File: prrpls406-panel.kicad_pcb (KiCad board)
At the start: 2 copper layers, 36 x 36 mm, 384 parts, among them U1 ATtiny406-M

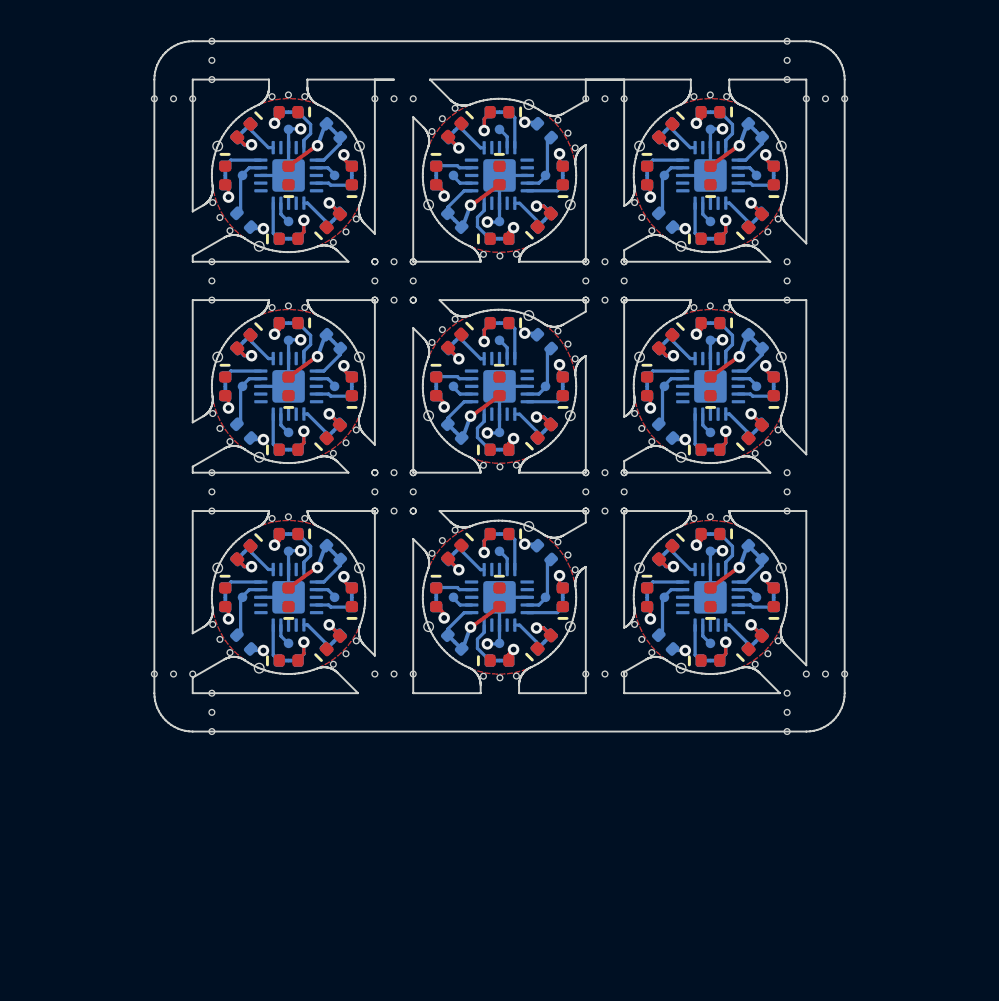
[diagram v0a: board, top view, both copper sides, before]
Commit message: submitting
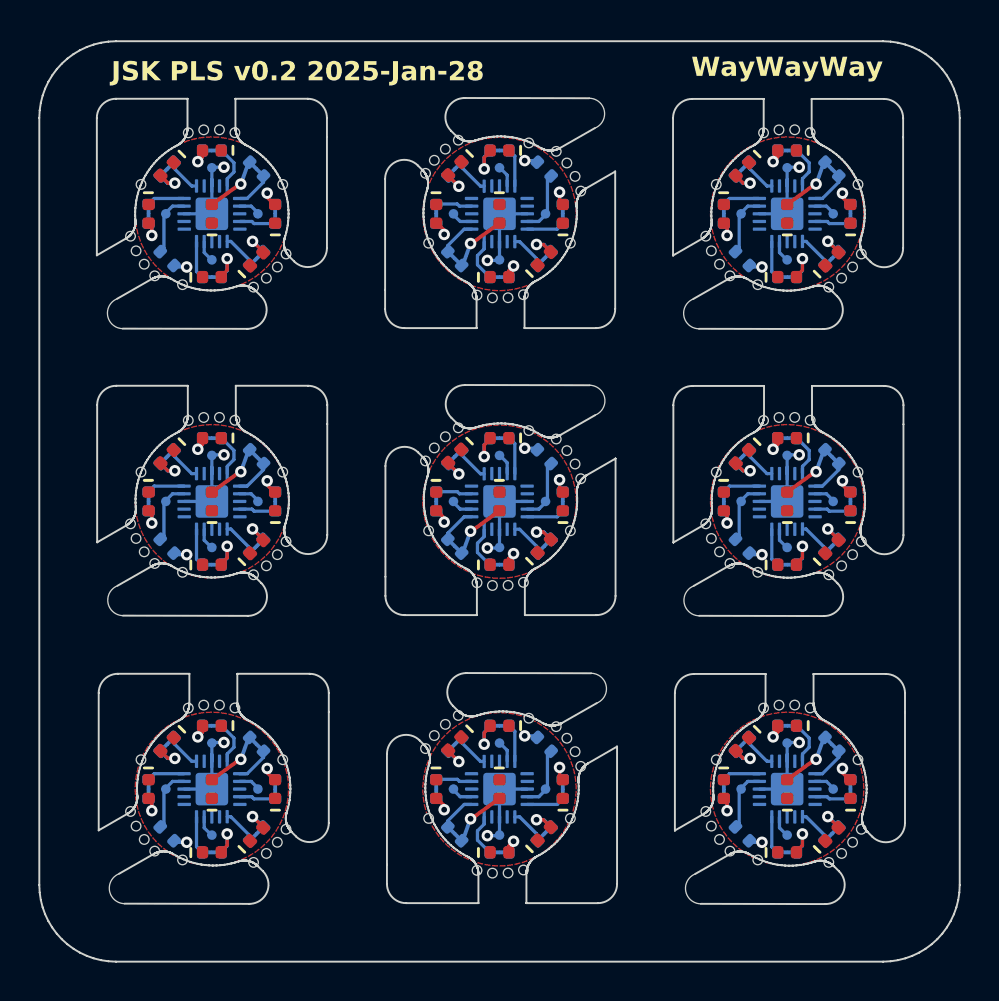
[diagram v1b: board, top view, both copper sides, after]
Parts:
- removed the C1 at (157.2, 40.3)
- removed the C1 at (150.8, 35.7)
- removed the C1 at (150.8, 46.7)
- removed the C1 at (157.2, 51.3)
- removed the C1 at (135.2, 29.3)
- removed the C1 at (135.2, 40.3)
- removed the C1 at (135.2, 51.3)
- removed the C1 at (150.8, 24.7)
- removed the C1 at (157.2, 29.3)
- removed the D1 at (159.5, 34.7)
- removed the D1 at (137.5, 34.7)
- removed the D1 at (148.5, 41.3)
- removed the D1 at (137.5, 45.7)
- removed the D1 at (159.5, 45.7)
- removed the D1 at (159.5, 23.7)
- removed the D1 at (137.5, 23.7)
- removed the D1 at (148.5, 30.3)
- removed the D1 at (148.5, 52.3)
- removed the D2 at (135.2, 24.7)
- removed the D2 at (157.2, 35.7)
- removed the D2 at (135.2, 35.7)
- removed the D2 at (157.2, 46.7)
- removed the D2 at (150.8, 40.3)
- removed the D2 at (157.2, 24.7)
- removed the D2 at (135.2, 46.7)
- removed the D2 at (150.8, 51.3)
- removed the D2 at (150.8, 29.3)
- removed the D3 at (134.2, 49.0)
- removed the D3 at (156.2, 27.0)
- removed the D3 at (156.2, 49.0)
- removed the D3 at (134.2, 38.0)
- removed the D3 at (134.2, 27.0)
- removed the D3 at (151.8, 49.0)
- removed the D3 at (151.8, 27.0)
- removed the D3 at (151.8, 38.0)
- removed the D3 at (156.2, 38.0)
- removed the D4 at (137.5, 38.0)
- removed the D4 at (137.5, 27.0)
- removed the D4 at (159.5, 27.0)
- removed the D4 at (148.5, 27.0)
- removed the D4 at (148.5, 49.0)
- removed the D4 at (159.5, 49.0)
- removed the D4 at (137.5, 49.0)
- removed the D4 at (148.5, 38.0)
- removed the D4 at (159.5, 38.0)
- removed the D5 at (137.5, 30.3)
- removed the D5 at (159.5, 41.3)
- removed the D5 at (159.5, 30.3)
- removed the D5 at (148.5, 34.7)
- removed the D5 at (148.5, 45.7)
- removed the D5 at (137.5, 52.3)
- removed the D5 at (159.5, 52.3)
- removed the D5 at (137.5, 41.3)
- removed the D5 at (148.5, 23.7)
- removed the D6 at (146.2, 46.6)
- removed the D6 at (161.8, 29.4)
- removed the D6 at (161.8, 51.4)
- removed the D6 at (146.2, 35.6)
- removed the D6 at (146.2, 24.6)
- removed the D6 at (139.8, 51.4)
- removed the D6 at (139.8, 29.4)
- removed the D6 at (139.8, 40.4)
- removed the D6 at (161.8, 40.4)
- removed the D7 at (140.8, 49.0)
- removed the D7 at (145.2, 49.0)
- removed the D7 at (162.8, 49.0)
- removed the D7 at (162.8, 38.0)
- removed the D7 at (145.2, 27.0)
- removed the D7 at (140.8, 38.0)
- removed the D7 at (140.8, 27.0)
- removed the D7 at (162.8, 27.0)
- removed the D7 at (145.2, 38.0)
- removed the H1 at (133.8, 25.5)
- removed the H1 at (155.8, 25.5)
- removed the H1 at (155.8, 36.5)
- removed the H1 at (133.8, 47.5)
- removed the H1 at (133.8, 36.5)
- removed the H1 at (152.2, 28.5)
- removed the H1 at (152.2, 39.5)
- removed the H1 at (152.2, 50.5)
- removed the H1 at (155.8, 47.5)
- removed the H2 at (158.0, 41.7)
- removed the H2 at (136.0, 30.7)
- removed the H2 at (150.0, 45.3)
- removed the H2 at (136.0, 41.7)
- removed the H2 at (158.0, 30.7)
- removed the H2 at (158.0, 52.7)
- removed the H2 at (150.0, 23.3)
- removed the H2 at (150.0, 34.3)
- removed the H2 at (136.0, 52.7)
- removed the H3 at (141.2, 47.5)
- removed the H3 at (141.2, 25.5)
- removed the H3 at (144.8, 50.5)
- removed the H3 at (144.8, 39.5)
- removed the H3 at (141.2, 36.5)
- removed the H3 at (144.8, 28.5)
- removed the H3 at (163.2, 36.5)
- removed the H3 at (163.2, 47.5)
- removed the H3 at (163.2, 25.5)
- removed KiKit_MB_28_1, KiKit_MB_28_2, KiKit_MB_28_3, KiKit_MB_29_1, KiKit_MB_29_2, KiKit_MB_29_3, KiKit_MB_30_1, KiKit_MB_30_2, KiKit_MB_30_3, KiKit_MB_31_1, KiKit_MB_31_2, KiKit_MB_31_3, KiKit_MB_32_1, KiKit_MB_32_2, KiKit_MB_32_3, KiKit_MB_33_1, KiKit_MB_33_2, KiKit_MB_33_3, KiKit_MB_34_1, KiKit_MB_34_2, KiKit_MB_34_3, KiKit_MB_35_1, KiKit_MB_35_2, KiKit_MB_35_3, KiKit_MB_36_1, KiKit_MB_36_2, KiKit_MB_36_3, KiKit_MB_37_1, KiKit_MB_37_2, KiKit_MB_37_3, KiKit_MB_38_1, KiKit_MB_38_2, KiKit_MB_38_3, KiKit_MB_39_1, KiKit_MB_39_2, KiKit_MB_39_3, KiKit_MB_40_1, KiKit_MB_40_2, KiKit_MB_40_3, KiKit_MB_41_1, KiKit_MB_41_2, KiKit_MB_41_3, KiKit_MB_42_1, KiKit_MB_42_2, KiKit_MB_42_3, KiKit_MB_43_1, KiKit_MB_43_2, KiKit_MB_43_3, KiKit_MB_44_1, KiKit_MB_44_2, KiKit_MB_44_3, KiKit_MB_45_1, KiKit_MB_45_2, KiKit_MB_45_3, KiKit_MB_46_1, KiKit_MB_46_2, KiKit_MB_46_3, KiKit_MB_47_1, KiKit_MB_47_2, KiKit_MB_47_3, KiKit_MB_48_1, KiKit_MB_48_2, KiKit_MB_48_3, KiKit_MB_49_1, KiKit_MB_49_2, KiKit_MB_49_3, KiKit_MB_50_1, KiKit_MB_50_2, KiKit_MB_50_3, KiKit_MB_51_1, KiKit_MB_51_2, KiKit_MB_51_3, KiKit_MB_52_1, KiKit_MB_52_2, KiKit_MB_52_3, KiKit_MB_53_1, KiKit_MB_53_2, KiKit_MB_53_3, KiKit_MB_54_1, KiKit_MB_54_2, KiKit_MB_54_3, KiKit_MB_55_1, KiKit_MB_55_2, KiKit_MB_55_3, KiKit_MB_56_1, KiKit_MB_56_2, KiKit_MB_56_3, KiKit_MB_57_1, KiKit_MB_57_2, KiKit_MB_57_3, KiKit_MB_58_1, KiKit_MB_58_2, KiKit_MB_58_3, KiKit_MB_59_1, KiKit_MB_59_2, KiKit_MB_59_3: NPTH, NPTH
- removed the R1 at (159.5, 45.7)
- removed the R1 at (159.5, 23.7)
- removed the R1 at (159.5, 34.7)
- removed the R1 at (148.5, 52.3)
- removed the R1 at (137.5, 34.7)
- removed the R1 at (137.5, 23.7)
- removed the R1 at (137.5, 45.7)
- removed the R1 at (148.5, 41.3)
- removed the R1 at (148.5, 30.3)
- removed the R2 at (150.8, 40.3)
- removed the R2 at (135.2, 24.7)
- removed the R2 at (157.2, 46.7)
- removed the R2 at (135.2, 46.7)
- removed the R2 at (150.8, 29.3)
- removed the R2 at (157.2, 24.7)
- removed the R2 at (157.2, 35.7)
- removed the R2 at (135.2, 35.7)
- removed the R2 at (150.8, 51.3)
- removed the R3 at (151.8, 27.0)
- removed the R3 at (151.8, 49.0)
- removed the R3 at (134.2, 27.0)
- removed the R3 at (156.2, 27.0)
- removed the R3 at (156.2, 38.0)
- removed the R3 at (134.2, 49.0)
- removed the R3 at (134.2, 38.0)
- removed the R3 at (151.8, 38.0)
- removed the R3 at (156.2, 49.0)
- removed the R4 at (161.8, 46.7)
- removed the R4 at (139.8, 24.7)
- removed the R4 at (161.8, 35.7)
- removed the R4 at (161.8, 24.7)
- removed the R4 at (139.8, 46.7)
- removed the R4 at (146.2, 51.3)
- removed the R4 at (139.8, 35.7)
- removed the R4 at (146.2, 29.3)
- removed the R4 at (146.2, 40.3)
- removed the R5 at (148.5, 34.7)
- removed the R5 at (159.5, 52.3)
- removed the R5 at (159.5, 30.3)
- removed the R5 at (159.5, 41.3)
- removed the R5 at (137.5, 52.3)
- removed the R5 at (137.5, 30.3)
- removed the R5 at (137.5, 41.3)
- removed the R5 at (148.5, 45.7)
- removed the R5 at (148.5, 23.7)
- removed the R6 at (161.8, 51.3)
- removed the R6 at (146.2, 24.7)
- removed the R6 at (161.8, 40.3)
- removed the R6 at (161.8, 29.3)
- removed the R6 at (146.2, 46.7)
- removed the R6 at (139.8, 51.3)
- removed the R6 at (146.2, 35.7)
- removed the R6 at (139.8, 29.3)
- removed the R6 at (139.8, 40.3)
- removed the R7 at (162.8, 49.0)
- removed the R7 at (140.8, 38.0)
- removed the R7 at (145.2, 49.0)
- removed the R7 at (145.2, 38.0)
- removed the R7 at (162.8, 27.0)
- removed the R7 at (162.8, 38.0)
- removed the R7 at (140.8, 27.0)
- removed the R7 at (140.8, 49.0)
- removed the R7 at (145.2, 27.0)
- removed the TP1 at (148.5, 40.4)
- removed the TP1 at (159.5, 46.6)
- removed the TP1 at (137.5, 35.6)
- removed the TP1 at (148.5, 29.4)
- removed the TP1 at (148.5, 51.4)
- removed the TP1 at (159.5, 35.6)
- removed the TP1 at (137.5, 46.6)
- removed the TP1 at (137.5, 24.6)
- removed the TP1 at (159.5, 24.6)
- removed the TP2 at (157.1, 38.0)
- removed the TP2 at (150.9, 27.0)
- removed the TP2 at (135.1, 27.0)
- removed the TP2 at (135.1, 38.0)
- removed the TP2 at (150.9, 38.0)
- removed the TP2 at (135.1, 49.0)
- removed the TP2 at (157.1, 49.0)
- removed the TP2 at (150.9, 49.0)
- removed the TP2 at (157.1, 27.0)
- removed the TP3 at (161.9, 27.0)
- removed the TP3 at (146.1, 27.0)
- removed the TP3 at (161.9, 38.0)
- removed the TP3 at (161.9, 49.0)
- removed the TP3 at (139.9, 38.0)
- removed the TP3 at (139.9, 27.0)
- removed the TP3 at (146.1, 49.0)
- removed the TP3 at (146.1, 38.0)
- removed the TP3 at (139.9, 49.0)
- removed the TP4 at (148.5, 35.6)
- removed the TP4 at (137.5, 40.4)
- removed the TP4 at (148.5, 24.6)
- removed the TP4 at (159.5, 51.4)
- removed the TP4 at (148.5, 46.6)
- removed the TP4 at (159.5, 40.4)
- removed the TP4 at (137.5, 51.4)
- removed the TP4 at (137.5, 29.4)
- removed the TP4 at (159.5, 29.4)
- removed the U1 at (159.5, 27.0)
- removed the U1 at (159.5, 38.0)
- removed the U1 at (148.5, 49.0)
- removed the U1 at (159.5, 49.0)
- removed the U1 at (148.5, 38.0)
- removed the U1 at (137.5, 27.0)
- removed the U1 at (137.5, 38.0)
- removed the U1 at (148.5, 27.0)
- removed the U1 at (137.5, 49.0)
- added C1: 0.1μF, JSK:R_0402_1005Metric_short_lines, B.Cu at (161.2, 31.3)
- added C1: 0.1μF, JSK:R_0402_1005Metric_short_lines, B.Cu at (150.8, 56.7)
- added C1: 0.1μF, JSK:R_0402_1005Metric_short_lines, B.Cu at (131.2, 31.3)
- added C1: 0.1μF, JSK:R_0402_1005Metric_short_lines, B.Cu at (150.8, 41.7)
- added C1: 0.1μF, JSK:R_0402_1005Metric_short_lines, B.Cu at (131.2, 46.3)
- added C1: 0.1μF, JSK:R_0402_1005Metric_short_lines, B.Cu at (150.8, 26.7)
- added C1: 0.1μF, JSK:R_0402_1005Metric_short_lines, B.Cu at (131.2, 61.3)
- added C1: 0.1μF, JSK:R_0402_1005Metric_short_lines, B.Cu at (161.2, 46.3)
- added C1: 0.1μF, JSK:R_0402_1005Metric_short_lines, B.Cu at (161.2, 61.3)
- added D1: LED_Small_Filled, JSK:LED_0402_1005Metric, F.Cu at (163.5, 55.7)
- added D1: LED_Small_Filled, JSK:LED_0402_1005Metric, F.Cu at (133.5, 25.7)
- added D1: LED_Small_Filled, JSK:LED_0402_1005Metric, F.Cu at (133.5, 55.7)
- added D1: LED_Small_Filled, JSK:LED_0402_1005Metric, F.Cu at (148.5, 32.3)
- added D1: LED_Small_Filled, JSK:LED_0402_1005Metric, F.Cu at (163.5, 40.7)
- added D1: LED_Small_Filled, JSK:LED_0402_1005Metric, F.Cu at (133.5, 40.7)
- added D1: LED_Small_Filled, JSK:LED_0402_1005Metric, F.Cu at (148.5, 47.3)
- added D1: LED_Small_Filled, JSK:LED_0402_1005Metric, F.Cu at (163.5, 25.7)
- added D1: LED_Small_Filled, JSK:LED_0402_1005Metric, F.Cu at (148.5, 62.3)
- added D2: LED_Small_Filled, JSK:LED_0402_1005Metric, F.Cu at (161.2, 56.7)
- added D2: LED_Small_Filled, JSK:LED_0402_1005Metric, F.Cu at (150.8, 61.3)
- added D2: LED_Small_Filled, JSK:LED_0402_1005Metric, F.Cu at (161.2, 41.7)
- added D2: LED_Small_Filled, JSK:LED_0402_1005Metric, F.Cu at (161.2, 26.7)
- added D2: LED_Small_Filled, JSK:LED_0402_1005Metric, F.Cu at (131.2, 26.7)
- added D2: LED_Small_Filled, JSK:LED_0402_1005Metric, F.Cu at (131.2, 41.7)
- added D2: LED_Small_Filled, JSK:LED_0402_1005Metric, F.Cu at (150.8, 46.3)
- added D2: LED_Small_Filled, JSK:LED_0402_1005Metric, F.Cu at (131.2, 56.7)
- added D2: LED_Small_Filled, JSK:LED_0402_1005Metric, F.Cu at (150.8, 31.3)
- added D3: LED_Small_Filled, JSK:LED_0402_1005Metric, F.Cu at (160.2, 59.0)
- added D3: LED_Small_Filled, JSK:LED_0402_1005Metric, F.Cu at (160.2, 44.0)
- added D3: LED_Small_Filled, JSK:LED_0402_1005Metric, F.Cu at (130.2, 29.0)
- added D3: LED_Small_Filled, JSK:LED_0402_1005Metric, F.Cu at (151.8, 29.0)
- added D3: LED_Small_Filled, JSK:LED_0402_1005Metric, F.Cu at (151.8, 59.0)
- added D3: LED_Small_Filled, JSK:LED_0402_1005Metric, F.Cu at (130.2, 59.0)
- added D3: LED_Small_Filled, JSK:LED_0402_1005Metric, F.Cu at (130.2, 44.0)
- added D3: LED_Small_Filled, JSK:LED_0402_1005Metric, F.Cu at (151.8, 44.0)
- added D3: LED_Small_Filled, JSK:LED_0402_1005Metric, F.Cu at (160.2, 29.0)
- added D4: LED_Small_Filled, JSK:LED_0402_1005Metric, F.Cu at (148.5, 44.0)
- added D4: LED_Small_Filled, JSK:LED_0402_1005Metric, F.Cu at (148.5, 29.0)
- added D4: LED_Small_Filled, JSK:LED_0402_1005Metric, F.Cu at (163.5, 44.0)
- added D4: LED_Small_Filled, JSK:LED_0402_1005Metric, F.Cu at (163.5, 59.0)
- added D4: LED_Small_Filled, JSK:LED_0402_1005Metric, F.Cu at (163.5, 29.0)
- added D4: LED_Small_Filled, JSK:LED_0402_1005Metric, F.Cu at (133.5, 29.0)
- added D4: LED_Small_Filled, JSK:LED_0402_1005Metric, F.Cu at (148.5, 59.0)
- added D4: LED_Small_Filled, JSK:LED_0402_1005Metric, F.Cu at (133.5, 44.0)
- added D4: LED_Small_Filled, JSK:LED_0402_1005Metric, F.Cu at (133.5, 59.0)
- added D5: LED_Small_Filled, JSK:LED_0402_1005Metric, F.Cu at (163.5, 62.3)
- added D5: LED_Small_Filled, JSK:LED_0402_1005Metric, F.Cu at (148.5, 25.7)
- added D5: LED_Small_Filled, JSK:LED_0402_1005Metric, F.Cu at (133.5, 32.3)
- added D5: LED_Small_Filled, JSK:LED_0402_1005Metric, F.Cu at (133.5, 62.3)
- added D5: LED_Small_Filled, JSK:LED_0402_1005Metric, F.Cu at (148.5, 40.7)
- added D5: LED_Small_Filled, JSK:LED_0402_1005Metric, F.Cu at (148.5, 55.7)
- added D5: LED_Small_Filled, JSK:LED_0402_1005Metric, F.Cu at (163.5, 32.3)
- added D5: LED_Small_Filled, JSK:LED_0402_1005Metric, F.Cu at (133.5, 47.3)
- added D5: LED_Small_Filled, JSK:LED_0402_1005Metric, F.Cu at (163.5, 47.3)
- added D6: LED_Small_Filled, JSK:LED_0402_1005Metric, F.Cu at (165.8, 46.4)
- added D6: LED_Small_Filled, JSK:LED_0402_1005Metric, F.Cu at (165.8, 61.4)
- added D6: LED_Small_Filled, JSK:LED_0402_1005Metric, F.Cu at (135.8, 46.4)
- added D6: LED_Small_Filled, JSK:LED_0402_1005Metric, F.Cu at (135.8, 61.4)
- added D6: LED_Small_Filled, JSK:LED_0402_1005Metric, F.Cu at (135.8, 31.4)
- added D6: LED_Small_Filled, JSK:LED_0402_1005Metric, F.Cu at (165.8, 31.4)
- added D6: LED_Small_Filled, JSK:LED_0402_1005Metric, F.Cu at (146.2, 41.6)
- added D6: LED_Small_Filled, JSK:LED_0402_1005Metric, F.Cu at (146.2, 56.6)
- added D6: LED_Small_Filled, JSK:LED_0402_1005Metric, F.Cu at (146.2, 26.6)
- added D7: LED_Small_Filled, JSK:LED_0402_1005Metric, F.Cu at (145.2, 29.0)
- added D7: LED_Small_Filled, JSK:LED_0402_1005Metric, F.Cu at (145.2, 59.0)
- added D7: LED_Small_Filled, JSK:LED_0402_1005Metric, F.Cu at (145.2, 44.0)
- added D7: LED_Small_Filled, JSK:LED_0402_1005Metric, F.Cu at (166.8, 44.0)
- added D7: LED_Small_Filled, JSK:LED_0402_1005Metric, F.Cu at (136.8, 44.0)
- added D7: LED_Small_Filled, JSK:LED_0402_1005Metric, F.Cu at (166.8, 29.0)
- added D7: LED_Small_Filled, JSK:LED_0402_1005Metric, F.Cu at (136.8, 59.0)
- added D7: LED_Small_Filled, JSK:LED_0402_1005Metric, F.Cu at (166.8, 59.0)
- added D7: LED_Small_Filled, JSK:LED_0402_1005Metric, F.Cu at (136.8, 29.0)
- added H1: MountingHole, JSK:0.5 npth, F.Cu at (152.2, 30.5)
- added H1: MountingHole, JSK:0.5 npth, F.Cu at (152.2, 45.5)
- added H1: MountingHole, JSK:0.5 npth, F.Cu at (129.8, 57.5)
- added H1: MountingHole, JSK:0.5 npth, F.Cu at (129.8, 27.5)
- added H1: MountingHole, JSK:0.5 npth, F.Cu at (159.8, 57.5)
- added H1: MountingHole, JSK:0.5 npth, F.Cu at (159.8, 42.5)
- added H1: MountingHole, JSK:0.5 npth, F.Cu at (159.8, 27.5)
- added H1: MountingHole, JSK:0.5 npth, F.Cu at (152.2, 60.5)
- added H1: MountingHole, JSK:0.5 npth, F.Cu at (129.8, 42.5)
- added H2: MountingHole, JSK:0.5 npth, F.Cu at (150.0, 40.3)
- added H2: MountingHole, JSK:0.5 npth, F.Cu at (132.0, 47.7)
- added H2: MountingHole, JSK:0.5 npth, F.Cu at (132.0, 32.7)
- added H2: MountingHole, JSK:0.5 npth, F.Cu at (150.0, 25.3)
- added H2: MountingHole, JSK:0.5 npth, F.Cu at (150.0, 55.3)
- added H2: MountingHole, JSK:0.5 npth, F.Cu at (132.0, 62.7)
- added H2: MountingHole, JSK:0.5 npth, F.Cu at (162.0, 32.7)
- added H2: MountingHole, JSK:0.5 npth, F.Cu at (162.0, 62.7)
- added H2: MountingHole, JSK:0.5 npth, F.Cu at (162.0, 47.7)
- added H3: MountingHole, JSK:0.5 npth, F.Cu at (167.2, 57.5)
- added H3: MountingHole, JSK:0.5 npth, F.Cu at (144.8, 45.5)
- added H3: MountingHole, JSK:0.5 npth, F.Cu at (167.2, 42.5)
- added H3: MountingHole, JSK:0.5 npth, F.Cu at (137.2, 27.5)
- added H3: MountingHole, JSK:0.5 npth, F.Cu at (144.8, 30.5)
- added H3: MountingHole, JSK:0.5 npth, F.Cu at (167.2, 27.5)
- added H3: MountingHole, JSK:0.5 npth, F.Cu at (137.2, 57.5)
- added H3: MountingHole, JSK:0.5 npth, F.Cu at (137.2, 42.5)
- added H3: MountingHole, JSK:0.5 npth, F.Cu at (144.8, 60.5)
- added KiKit_MB_10_5: NPTH, NPTH, F.Cu at (129.3, 45.2)
- added KiKit_MB_11_5: NPTH, NPTH, F.Cu at (135.7, 47.8)
- added KiKit_MB_12_5: NPTH, NPTH, F.Cu at (134.7, 39.8)
- added KiKit_MB_13_5: NPTH, NPTH, F.Cu at (152.7, 42.8)
- added KiKit_MB_14_5: NPTH, NPTH, F.Cu at (146.4, 40.2)
- added KiKit_MB_15_5: NPTH, NPTH, F.Cu at (147.3, 48.2)
- added KiKit_MB_16_5: NPTH, NPTH, F.Cu at (159.3, 45.2)
- added KiKit_MB_17_5: NPTH, NPTH, F.Cu at (165.7, 47.8)
- added KiKit_MB_18_5: NPTH, NPTH, F.Cu at (164.7, 39.8)
- added KiKit_MB_19_5: NPTH, NPTH, F.Cu at (129.3, 60.2)
- added KiKit_MB_1_5: NPTH, NPTH, F.Cu at (129.3, 30.2)
- added KiKit_MB_20_5: NPTH, NPTH, F.Cu at (135.7, 62.8)
- added KiKit_MB_21_5: NPTH, NPTH, F.Cu at (134.7, 54.8)
- added KiKit_MB_22_5: NPTH, NPTH, F.Cu at (152.7, 57.8)
- added KiKit_MB_23_5: NPTH, NPTH, F.Cu at (146.4, 55.2)
- added KiKit_MB_24_5: NPTH, NPTH, F.Cu at (147.3, 63.2)
- added KiKit_MB_25_5: NPTH, NPTH, F.Cu at (159.3, 60.2)
- added KiKit_MB_26_5: NPTH, NPTH, F.Cu at (165.7, 62.8)
- added KiKit_MB_27_5: NPTH, NPTH, F.Cu at (164.7, 54.8)
- added KiKit_MB_2_5: NPTH, NPTH, F.Cu at (135.7, 32.8)
- added KiKit_MB_3_5: NPTH, NPTH, F.Cu at (134.7, 24.8)
- added KiKit_MB_4_5: NPTH, NPTH, F.Cu at (152.7, 27.8)
- added KiKit_MB_5_5: NPTH, NPTH, F.Cu at (146.4, 25.2)
- added KiKit_MB_6_5: NPTH, NPTH, F.Cu at (147.3, 33.2)
- added KiKit_MB_7_5: NPTH, NPTH, F.Cu at (159.3, 30.2)
- added KiKit_MB_8_5: NPTH, NPTH, F.Cu at (165.7, 32.8)
- added KiKit_MB_9_5: NPTH, NPTH, F.Cu at (164.7, 24.8)
- added R1: 0, JSK:Jumpered_R_0402_1005Metric, B.Cu at (163.5, 25.7)
- added R1: 0, JSK:Jumpered_R_0402_1005Metric, B.Cu at (163.5, 55.7)
- added R1: 0, JSK:Jumpered_R_0402_1005Metric, B.Cu at (148.5, 62.3)
- added R1: 0, JSK:Jumpered_R_0402_1005Metric, B.Cu at (133.5, 55.7)
- added R1: 0, JSK:Jumpered_R_0402_1005Metric, B.Cu at (163.5, 40.7)
- added R1: 0, JSK:Jumpered_R_0402_1005Metric, B.Cu at (133.5, 25.7)
- added R1: 0, JSK:Jumpered_R_0402_1005Metric, B.Cu at (148.5, 32.3)
- added R1: 0, JSK:Jumpered_R_0402_1005Metric, B.Cu at (148.5, 47.3)
- added R1: 0, JSK:Jumpered_R_0402_1005Metric, B.Cu at (133.5, 40.7)
- added R2: 0, JSK:Jumpered_R_0402_1005Metric, B.Cu at (131.2, 26.7)
- added R2: 0, JSK:Jumpered_R_0402_1005Metric, B.Cu at (150.8, 31.3)
- added R2: 0, JSK:Jumpered_R_0402_1005Metric, B.Cu at (161.2, 26.7)
- added R2: 0, JSK:Jumpered_R_0402_1005Metric, B.Cu at (131.2, 56.7)
- added R2: 0, JSK:Jumpered_R_0402_1005Metric, B.Cu at (150.8, 46.3)
- added R2: 0, JSK:Jumpered_R_0402_1005Metric, B.Cu at (161.2, 56.7)
- added R2: 0, JSK:Jumpered_R_0402_1005Metric, B.Cu at (161.2, 41.7)
- added R2: 0, JSK:Jumpered_R_0402_1005Metric, B.Cu at (150.8, 61.3)
- added R2: 0, JSK:Jumpered_R_0402_1005Metric, B.Cu at (131.2, 41.7)
- added R3: 0, JSK:Jumpered_R_0402_1005Metric, B.Cu at (151.8, 29.0)
- added R3: 0, JSK:Jumpered_R_0402_1005Metric, B.Cu at (160.2, 59.0)
- added R3: 0, JSK:Jumpered_R_0402_1005Metric, B.Cu at (151.8, 44.0)
- added R3: 0, JSK:Jumpered_R_0402_1005Metric, B.Cu at (130.2, 59.0)
- added R3: 0, JSK:Jumpered_R_0402_1005Metric, B.Cu at (130.2, 29.0)
- added R3: 0, JSK:Jumpered_R_0402_1005Metric, B.Cu at (160.2, 29.0)
- added R3: 0, JSK:Jumpered_R_0402_1005Metric, B.Cu at (151.8, 59.0)
- added R3: 0, JSK:Jumpered_R_0402_1005Metric, B.Cu at (160.2, 44.0)
- added R3: 0, JSK:Jumpered_R_0402_1005Metric, B.Cu at (130.2, 44.0)
- added R4: 0, JSK:Jumpered_R_0402_1005Metric, B.Cu at (165.8, 26.7)
- added R4: 0, JSK:Jumpered_R_0402_1005Metric, B.Cu at (135.8, 26.7)
- added R4: 0, JSK:Jumpered_R_0402_1005Metric, B.Cu at (146.2, 31.3)
- added R4: 0, JSK:Jumpered_R_0402_1005Metric, B.Cu at (165.8, 56.7)
- added R4: 0, JSK:Jumpered_R_0402_1005Metric, B.Cu at (135.8, 56.7)
- added R4: 0, JSK:Jumpered_R_0402_1005Metric, B.Cu at (165.8, 41.7)
- added R4: 0, JSK:Jumpered_R_0402_1005Metric, B.Cu at (135.8, 41.7)
- added R4: 0, JSK:Jumpered_R_0402_1005Metric, B.Cu at (146.2, 46.3)
- added R4: 0, JSK:Jumpered_R_0402_1005Metric, B.Cu at (146.2, 61.3)
- added R5: 0, JSK:Jumpered_R_0402_1005Metric, B.Cu at (133.5, 47.3)
- added R5: 0, JSK:Jumpered_R_0402_1005Metric, B.Cu at (163.5, 47.3)
- added R5: 0, JSK:Jumpered_R_0402_1005Metric, B.Cu at (148.5, 55.7)
- added R5: 0, JSK:Jumpered_R_0402_1005Metric, B.Cu at (148.5, 40.7)
- added R5: 0, JSK:Jumpered_R_0402_1005Metric, B.Cu at (133.5, 62.3)
- added R5: 0, JSK:Jumpered_R_0402_1005Metric, B.Cu at (133.5, 32.3)
- added R5: 0, JSK:Jumpered_R_0402_1005Metric, B.Cu at (148.5, 25.7)
- added R5: 0, JSK:Jumpered_R_0402_1005Metric, B.Cu at (163.5, 62.3)
- added R5: 0, JSK:Jumpered_R_0402_1005Metric, B.Cu at (163.5, 32.3)
- added R6: 0, JSK:Jumpered_R_0402_1005Metric, B.Cu at (135.8, 46.3)
- added R6: 0, JSK:Jumpered_R_0402_1005Metric, B.Cu at (165.8, 61.3)
- added R6: 0, JSK:Jumpered_R_0402_1005Metric, B.Cu at (146.2, 56.7)
- added R6: 0, JSK:Jumpered_R_0402_1005Metric, B.Cu at (146.2, 26.7)
- added R6: 0, JSK:Jumpered_R_0402_1005Metric, B.Cu at (135.8, 31.3)
- added R6: 0, JSK:Jumpered_R_0402_1005Metric, B.Cu at (135.8, 61.3)
- added R6: 0, JSK:Jumpered_R_0402_1005Metric, B.Cu at (146.2, 41.7)
- added R6: 0, JSK:Jumpered_R_0402_1005Metric, B.Cu at (165.8, 46.3)
- added R6: 0, JSK:Jumpered_R_0402_1005Metric, B.Cu at (165.8, 31.3)
- added R7: 0, JSK:Jumpered_R_0402_1005Metric, B.Cu at (136.8, 29.0)
- added R7: 0, JSK:Jumpered_R_0402_1005Metric, B.Cu at (166.8, 44.0)
- added R7: 0, JSK:Jumpered_R_0402_1005Metric, B.Cu at (136.8, 44.0)
- added R7: 0, JSK:Jumpered_R_0402_1005Metric, B.Cu at (166.8, 29.0)
- added R7: 0, JSK:Jumpered_R_0402_1005Metric, B.Cu at (136.8, 59.0)
- added R7: 0, JSK:Jumpered_R_0402_1005Metric, B.Cu at (145.2, 59.0)
- added R7: 0, JSK:Jumpered_R_0402_1005Metric, B.Cu at (145.2, 29.0)
- added R7: 0, JSK:Jumpered_R_0402_1005Metric, B.Cu at (145.2, 44.0)
- added R7: 0, JSK:Jumpered_R_0402_1005Metric, B.Cu at (166.8, 59.0)
- added TP1: TestPoint, JSK:0.5mm-pogo-pad, B.Cu at (133.5, 56.6)
- added TP1: TestPoint, JSK:0.5mm-pogo-pad, B.Cu at (148.5, 46.4)
- added TP1: TestPoint, JSK:0.5mm-pogo-pad, B.Cu at (133.5, 41.6)
- added TP1: TestPoint, JSK:0.5mm-pogo-pad, B.Cu at (148.5, 61.4)
- added TP1: TestPoint, JSK:0.5mm-pogo-pad, B.Cu at (163.5, 41.6)
- added TP1: TestPoint, JSK:0.5mm-pogo-pad, B.Cu at (133.5, 26.6)
- added TP1: TestPoint, JSK:0.5mm-pogo-pad, B.Cu at (163.5, 56.6)
- added TP1: TestPoint, JSK:0.5mm-pogo-pad, B.Cu at (148.5, 31.4)
- added TP1: TestPoint, JSK:0.5mm-pogo-pad, B.Cu at (163.5, 26.6)
- added TP2: TestPoint, JSK:0.5mm-pogo-pad, B.Cu at (161.1, 44.0)
- added TP2: TestPoint, JSK:0.5mm-pogo-pad, B.Cu at (150.9, 44.0)
- added TP2: TestPoint, JSK:0.5mm-pogo-pad, B.Cu at (161.1, 29.0)
- added TP2: TestPoint, JSK:0.5mm-pogo-pad, B.Cu at (131.1, 44.0)
- added TP2: TestPoint, JSK:0.5mm-pogo-pad, B.Cu at (131.1, 59.0)
- added TP2: TestPoint, JSK:0.5mm-pogo-pad, B.Cu at (161.1, 59.0)
- added TP2: TestPoint, JSK:0.5mm-pogo-pad, B.Cu at (150.9, 29.0)
- added TP2: TestPoint, JSK:0.5mm-pogo-pad, B.Cu at (150.9, 59.0)
- added TP2: TestPoint, JSK:0.5mm-pogo-pad, B.Cu at (131.1, 29.0)
- added TP3: TestPoint, JSK:0.5mm-pogo-pad, B.Cu at (165.9, 59.0)
- added TP3: TestPoint, JSK:0.5mm-pogo-pad, B.Cu at (135.9, 29.0)
- added TP3: TestPoint, JSK:0.5mm-pogo-pad, B.Cu at (135.9, 59.0)
- added TP3: TestPoint, JSK:0.5mm-pogo-pad, B.Cu at (135.9, 44.0)
- added TP3: TestPoint, JSK:0.5mm-pogo-pad, B.Cu at (146.1, 59.0)
- added TP3: TestPoint, JSK:0.5mm-pogo-pad, B.Cu at (146.1, 44.0)
- added TP3: TestPoint, JSK:0.5mm-pogo-pad, B.Cu at (146.1, 29.0)
- added TP3: TestPoint, JSK:0.5mm-pogo-pad, B.Cu at (165.9, 44.0)
- added TP3: TestPoint, JSK:0.5mm-pogo-pad, B.Cu at (165.9, 29.0)
- added TP4: TestPoint, JSK:0.5mm-pogo-pad, B.Cu at (133.5, 61.4)
- added TP4: TestPoint, JSK:0.5mm-pogo-pad, B.Cu at (163.5, 46.4)
- added TP4: TestPoint, JSK:0.5mm-pogo-pad, B.Cu at (148.5, 26.6)
- added TP4: TestPoint, JSK:0.5mm-pogo-pad, B.Cu at (133.5, 31.4)
- added TP4: TestPoint, JSK:0.5mm-pogo-pad, B.Cu at (148.5, 56.6)
- added TP4: TestPoint, JSK:0.5mm-pogo-pad, B.Cu at (163.5, 61.4)
- added TP4: TestPoint, JSK:0.5mm-pogo-pad, B.Cu at (163.5, 31.4)
- added TP4: TestPoint, JSK:0.5mm-pogo-pad, B.Cu at (133.5, 46.4)
- added TP4: TestPoint, JSK:0.5mm-pogo-pad, B.Cu at (148.5, 41.6)
- added U1: ATtiny406-M, JSK:extra_clearence_VQFN-20-1EP_3x3mm_P0.4mm_EP1.7x1.7mm, B.Cu at (148.5, 59.0)
- added U1: ATtiny406-M, JSK:extra_clearence_VQFN-20-1EP_3x3mm_P0.4mm_EP1.7x1.7mm, B.Cu at (133.5, 44.0)
- added U1: ATtiny406-M, JSK:extra_clearence_VQFN-20-1EP_3x3mm_P0.4mm_EP1.7x1.7mm, B.Cu at (163.5, 44.0)
- added U1: ATtiny406-M, JSK:extra_clearence_VQFN-20-1EP_3x3mm_P0.4mm_EP1.7x1.7mm, B.Cu at (133.5, 29.0)
- added U1: ATtiny406-M, JSK:extra_clearence_VQFN-20-1EP_3x3mm_P0.4mm_EP1.7x1.7mm, B.Cu at (148.5, 29.0)
- added U1: ATtiny406-M, JSK:extra_clearence_VQFN-20-1EP_3x3mm_P0.4mm_EP1.7x1.7mm, B.Cu at (163.5, 29.0)
- added U1: ATtiny406-M, JSK:extra_clearence_VQFN-20-1EP_3x3mm_P0.4mm_EP1.7x1.7mm, B.Cu at (148.5, 44.0)
- added U1: ATtiny406-M, JSK:extra_clearence_VQFN-20-1EP_3x3mm_P0.4mm_EP1.7x1.7mm, B.Cu at (133.5, 59.0)
- added U1: ATtiny406-M, JSK:extra_clearence_VQFN-20-1EP_3x3mm_P0.4mm_EP1.7x1.7mm, B.Cu at (163.5, 59.0)
- moved KiKit_MB_25_4 11.3 mm to (159.5, 60.9)
- moved KiKit_MB_19_4 11.3 mm to (129.5, 60.9)
- moved KiKit_MB_25_3 11.2 mm to (160.0, 61.6)
- moved KiKit_MB_19_3 11.2 mm to (130.0, 61.6)
- moved KiKit_MB_25_2 11.1 mm to (160.5, 62.2)
- moved KiKit_MB_19_2 11.1 mm to (130.5, 62.2)
- moved KiKit_MB_26_4 10.8 mm to (166.3, 62.4)
- moved KiKit_MB_21_2 10.8 mm to (132.3, 54.8)
- moved KiKit_MB_26_3 10.8 mm to (166.9, 61.8)
- moved KiKit_MB_21_3 10.8 mm to (133.1, 54.6)
- moved KiKit_MB_26_2 10.7 mm to (167.4, 61.1)
- moved KiKit_MB_21_4 10.7 mm to (133.9, 54.6)
- moved KiKit_MB_27_2 10.5 mm to (162.3, 54.8)
- moved KiKit_MB_20_2 10.5 mm to (137.4, 61.1)
- moved KiKit_MB_20_4 10.5 mm to (136.3, 62.4)
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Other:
- board size 36 x 36 mm -> 48 x 48 mm
- board text added: "JSK PLS v0.2 2025-Jan-28"
- board text added: "WayWayWay"
